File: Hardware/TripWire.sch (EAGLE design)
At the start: 50 parts, among them P1 LSP11, P2 LSP11, P3 LSP11, P4 LSP11, P5 LSP11, P6 LSP11, P7 LSP11, X1 GADGETEER-SOCKET

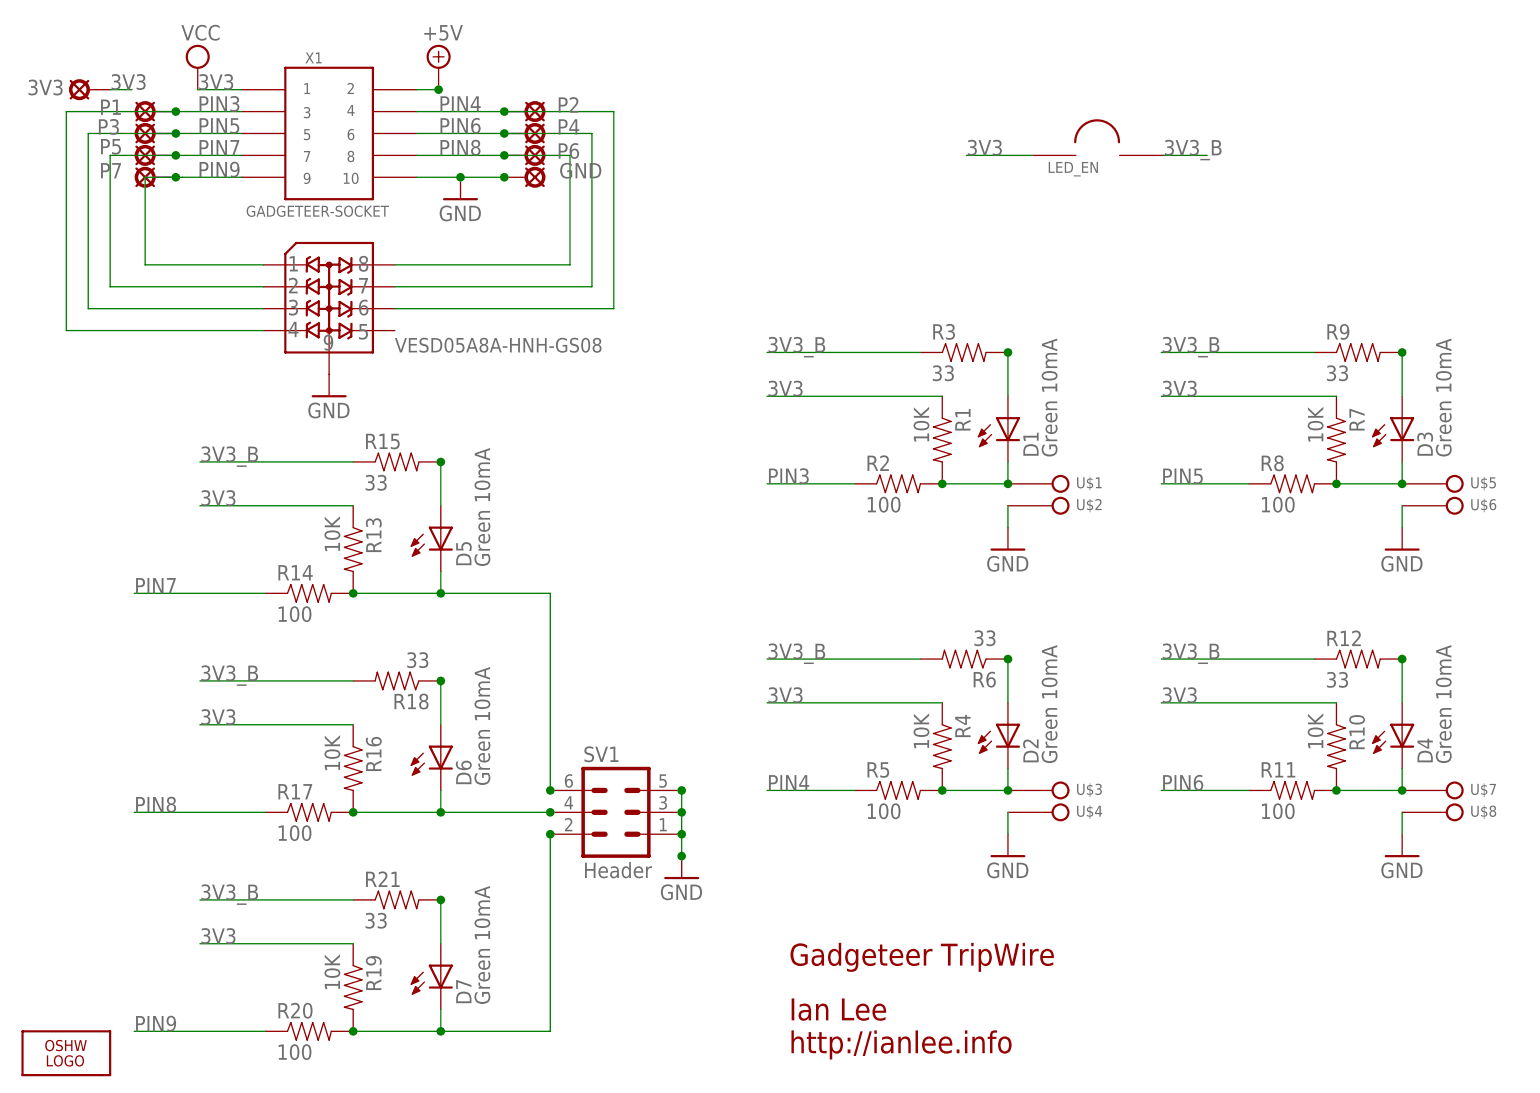
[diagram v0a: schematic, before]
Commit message: Changed the OSHW logo to use the SparkFun medium one.
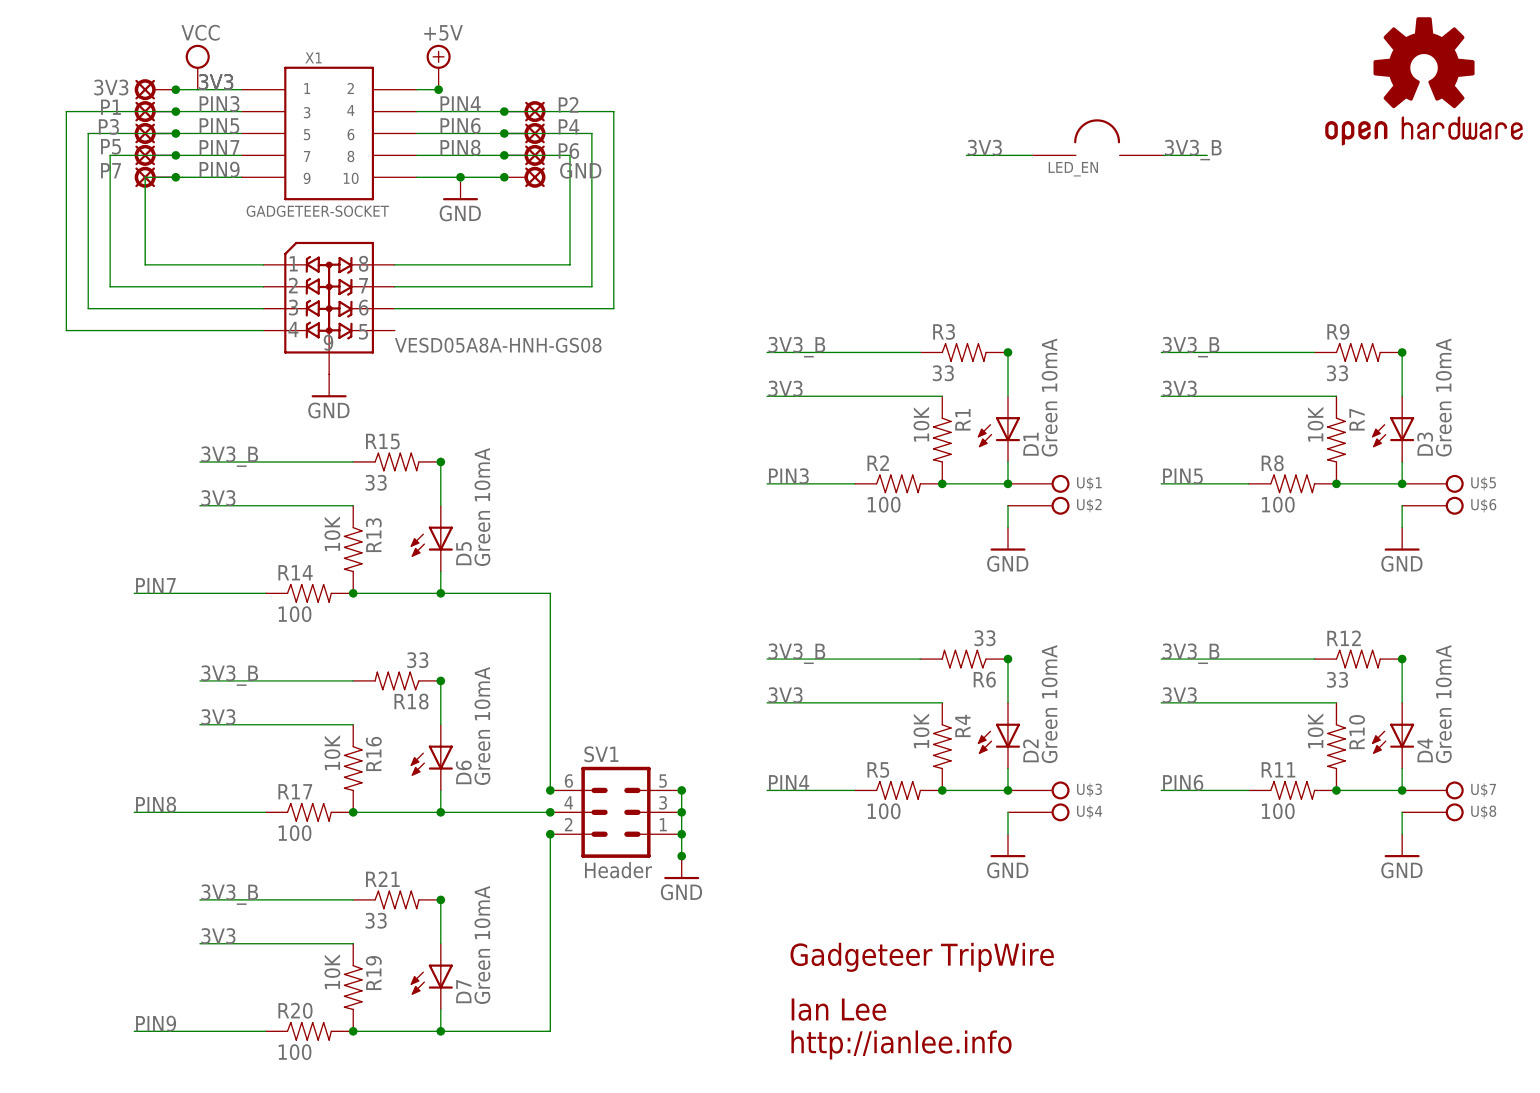
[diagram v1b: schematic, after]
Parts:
- LOGO1: value LOGO-OSHW-FILLX0200-NT -> OSHW-LOGOM; device Logo:LOGO-OSHW-FILLX0200-NT -> SparkFun-Aesthetics:OSHW-LOGOM
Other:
- moved on the sheet: 3V3
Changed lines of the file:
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@@
 <part name="V2" library="supply2" deviceset="VCC" device=""/>
 <part name="X1" library="SoftDust" deviceset="GADGETEER-SOCKET" device=""/>
-<part name="LOGO1" library="Logo" deviceset="LOGO-OSHW-FILL" device="X0200-NT"/>
 <part name="U$1" library="SoftDust" deviceset="SPADE-TERMINAL" device="PTH"/>
 <part name="U$2" library="SoftDust" deviceset="SPADE-TERMINAL" device="PTH"/>
@@
 <part name="GND7" library="supply1" deviceset="GND" device=""/>
 <part name="SUPPLY1" library="supply2" deviceset="+5V" device=""/>
+<part name="LOGO1" library="SparkFun-Aesthetics" deviceset="OSHW-LOGO" device="M"/>
 </parts>
 <sheets>
@@
 <attribute name="VALUE" x="30.988" y="104.648" size="1.27" layer="96"/>
 </instance>
-<instance part="LOGO1" gate="G$1" x="10.16" y="7.62"/>
 <instance part="U$1" gate="G$1" x="119.38" y="73.66"/>
 <instance part="U$2" gate="G$1" x="119.38" y="71.12"/>
@@
 <attribute name="NAME" x="67.31" y="109.093" size="1.778" layer="95"/>
 </instance>
-<instance part="3V3" gate="1" x="12.7" y="119.38" smashed="yes" rot="R90">
-<attribute name="NAME" x="9.906" y="120.523" size="1.778" layer="95" rot="R180"/>
+<instance part="3V3" gate="1" x="20.32" y="119.38" smashed="yes" rot="R90">
+<attribute name="NAME" x="17.526" y="120.523" size="1.778" layer="95" rot="R180"/>
 </instance>
 <instance part="P1" gate="1" x="20.32" y="116.84" smashed="yes" rot="R90">
@@
 <instance part="GND7" gate="1" x="40.64" y="83.82"/>
 <instance part="SUPPLY1" gate="+5V" x="53.34" y="121.92"/>
+<instance part="LOGO1" gate="G$1" x="167.64" y="121.92"/>
 </instances>
 <busses>
@@
 <label x="25.4" y="119.38" size="1.778" layer="95"/>
 <wire x1="25.4" y1="119.38" x2="30.48" y2="119.38" width="0.1524" layer="91"/>
+<pinref part="3V3" gate="1" pin="MP"/>
+<label x="25.4" y="119.38" size="1.778" layer="95"/>
+<wire x1="22.86" y1="119.38" x2="25.4" y2="119.38" width="0.1524" layer="91"/>
+<junction x="22.86" y="119.38"/>
 </segment>
 <segment>
@@
 <label x="114.554" y="111.76" size="1.778" layer="95"/>
 </segment>
-<segment>
-<pinref part="3V3" gate="1" pin="MP"/>
-<wire x1="15.24" y1="119.38" x2="17.78" y2="119.38" width="0.1524" layer="91"/>
-<label x="15.24" y="119.38" size="1.778" layer="95"/>
-</segment>
 </net>
